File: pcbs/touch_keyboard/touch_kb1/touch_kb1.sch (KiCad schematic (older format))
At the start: 12 parts

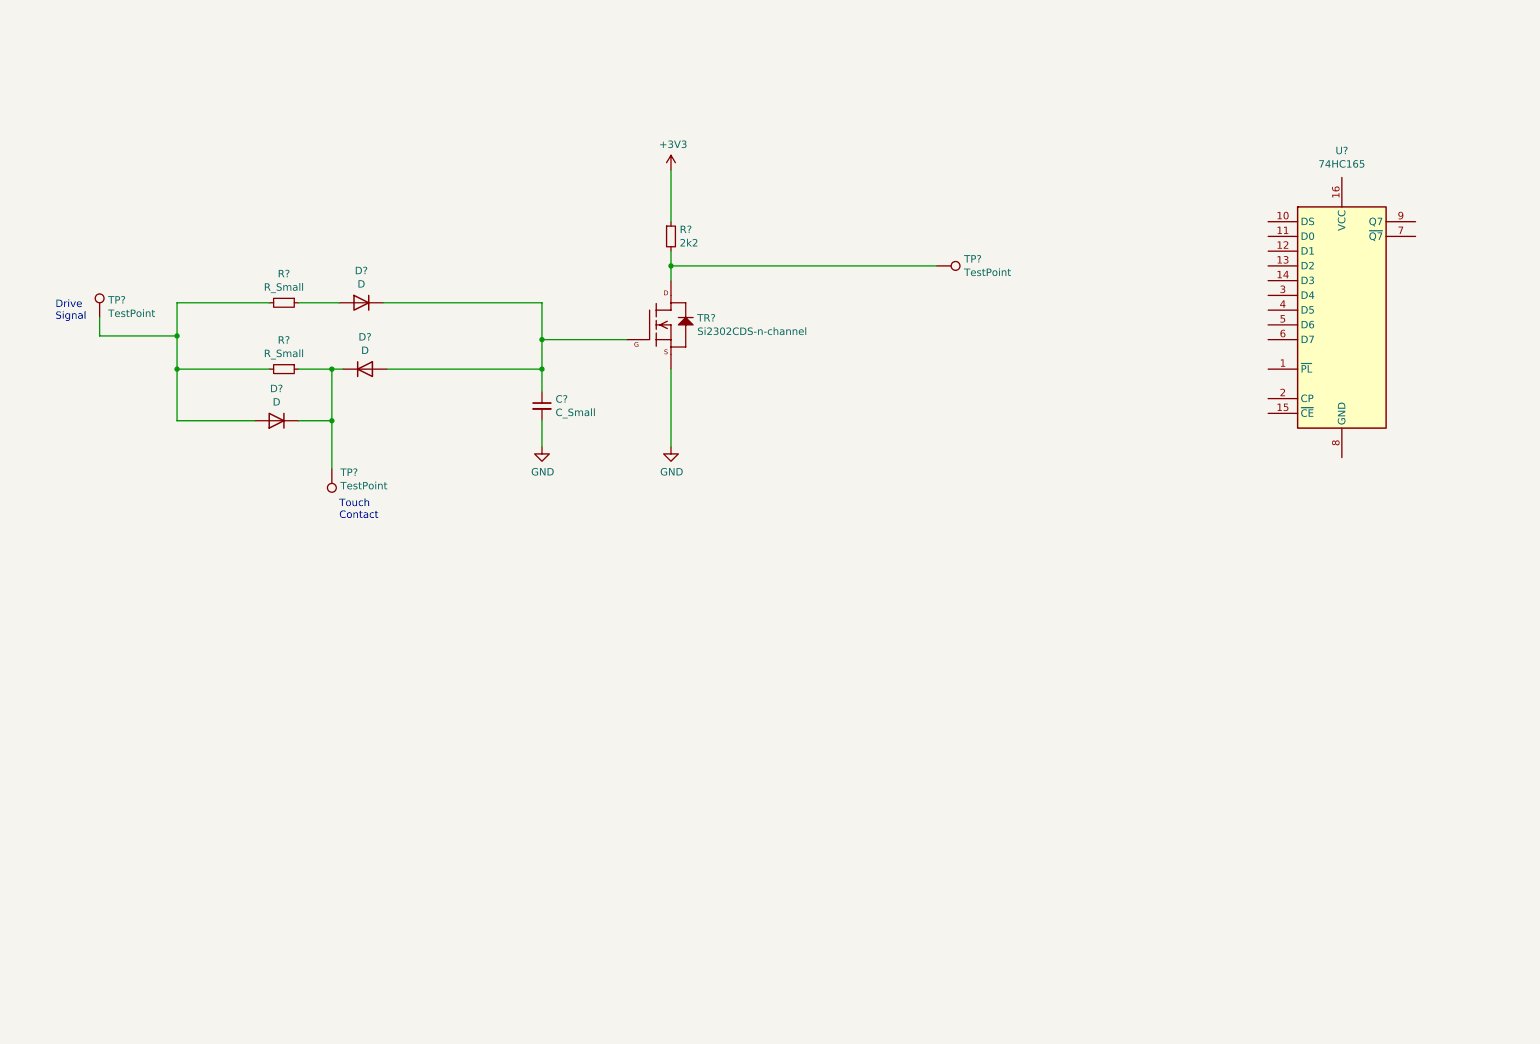
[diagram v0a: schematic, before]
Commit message: Updates
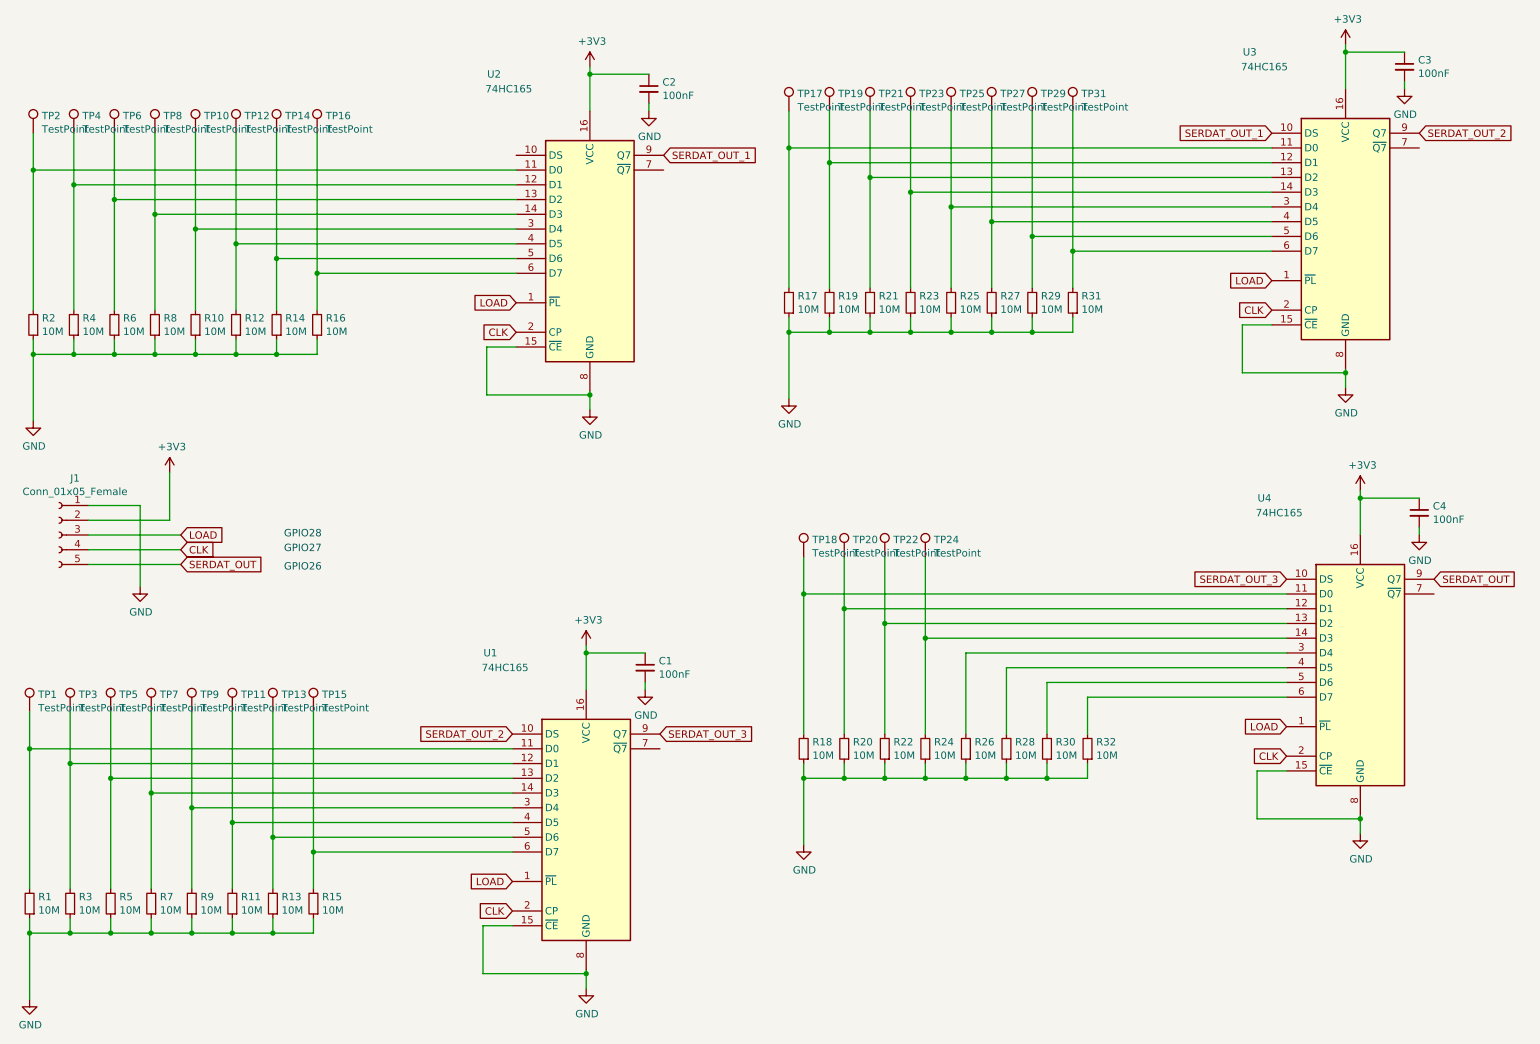
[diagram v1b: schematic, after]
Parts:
- removed C?: C_Small, symbol Device:C_Small
- removed D? (x3): D, symbol Device:D
- removed R? (x2): R_Small, symbol Device:R_Small
- removed TP? (x3): TestPoint, symbol Connector:TestPoint
- removed TR?: Si2302CDS-n-channel, Package_TO_SOT_SMD:SOT-23, symbol New_Library:Si2302CDS-n-channel
- added C1, C2, C3, C4: 100nF, Capacitor_SMD:C_0805_2012Metric_Pad1.18x1.45mm_HandSolder, symbol Device:C_Small
- added J1: Conn_01x05_Female, Connector_PinHeader_2.54mm:PinHeader_1x05_P2.54mm_Vertical_SMD_Pin1Left, symbol Connector:Conn_01x05_Female
- added R1, R10, R11, R12, R13, R14, R15, R16, R17, R18, R19, R2, R20, R21, R22, R23, R24, R25, R26, R27, R28, R29, R3, R30, R32, R4, R5, R6, R7, R8, R9: 10M, Resistor_SMD:R_0805_2012Metric_Pad1.20x1.40mm_HandSolder, symbol Device:R_Small
- added TP1, TP10, TP11, TP12, TP13, TP14, TP15, TP16, TP17, TP18, TP19, TP2, TP20, TP21, TP22, TP23, TP24, TP25, TP27, TP29, TP3, TP31, TP4, TP5, TP6, TP7, TP8, TP9: TestPoint, ajm_kicad:ESC_KB_Pad_half_size, symbol Connector:TestPoint
- added U1, U2, U4: 74HC165, Package_SO:SO-16_3.9x9.9mm_P1.27mm, symbol 74xx:74HC165
- R31: renamed from R?; value 2k2 -> 10M; footprint (none) -> Resistor_SMD:R_0805_2012Metric_Pad1.20x1.40mm_HandSolder
- U3: renamed from U?; footprint (none) -> Package_SO:SO-16_3.9x9.9mm_P1.27mm
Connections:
- net +3V3: now also U3.16 (VCC), C1.1, C2.1, C3.1, C4.1, J1.2 (Pin_2), U1.16 (VCC), U2.16 (VCC), U4.16 (VCC); no longer R31.1
- net GND: now also R31.1, U3.15 (~CE), U3.8 (GND), C1.2, C2.2, C3.2, C4.2, J1.1 (Pin_1), R1.1, R10.1, R11.1, R12.1, R13.1, R14.1, R15.1, R16.1, R17.1, R18.1, R19.1, R2.1, R20.1, R21.1, R22.1, R23.1, R24.1, R25.1, R26.1, R27.1, R28.1, R29.1, R3.1, R30.1, R32.1, R4.1, R5.1, R6.1, R7.1, R8.1, R9.1, U1.15 (~CE), U1.8 (GND), U2.15 (~CE), U2.8 (GND), U4.15 (~CE), U4.8 (GND)
- net at R31.2: now also U3.6 (D7), TP31.1
- net LOAD: now reaches U3.1 (~PL)
- net LOAD: now also J1.3 (Pin_3), U1.1 (~PL), U2.1 (~PL), U4.1 (~PL)
- net SERDAT_OUT_1: now reaches U3.10 (DS)
- net SERDAT_OUT_1: now also U2.9 (Q7)
- net at U3.11 (D0): now also R17.2, TP17.1
- net at U3.12 (D1): now also R19.2, TP19.1
- net at U3.13 (D2): now also R21.2, TP21.1
- net at U3.14 (D3): now also R23.2, TP23.1
- net CLK: now reaches U3.2 (CP)
- net CLK: now also J1.4 (Pin_4), U1.2 (CP), U2.2 (CP), U4.2 (CP)
- net at U3.3 (D4): now also R25.2, TP25.1
- net at U3.4 (D5): now also R27.2, TP27.1
- net at U3.5 (D6): now also R29.2, TP29.1
- net SERDAT_OUT_2: now reaches U3.9 (Q7)
- net SERDAT_OUT_2: now also U1.10 (DS)
- new net: R16.2, TP16.1, U2.6 (D7)
- new net: R2.2, TP2.1, U2.11 (D0)
- new net: R4.2, TP4.1, U2.12 (D1)
- new net: R6.2, TP6.1, U2.13 (D2)
- new net: R8.2, TP8.1, U2.14 (D3)
- new net: R10.2, TP10.1, U2.3 (D4)
- new net: R12.2, TP12.1, U2.4 (D5)
- new net: R14.2, TP14.1, U2.5 (D6)
- new net: R15.2, TP15.1, U1.6 (D7)
- new net: R1.2, TP1.1, U1.11 (D0)
- new net: R3.2, TP3.1, U1.12 (D1)
- new net: R5.2, TP5.1, U1.13 (D2)
- new net: R7.2, TP7.1, U1.14 (D3)
- new net: R9.2, TP9.1, U1.3 (D4)
- new net: R11.2, TP11.1, U1.4 (D5)
- new net: R13.2, TP13.1, U1.5 (D6)
- new net: R32.2, U4.6 (D7)
- new net: R18.2, TP18.1, U4.11 (D0)
- new net: R20.2, TP20.1, U4.12 (D1)
- new net: R22.2, TP22.1, U4.13 (D2)
- new net: R24.2, TP24.1, U4.14 (D3)
- new net: R26.2, U4.3 (D4)
- new net: R28.2, U4.4 (D5)
- new net: R30.2, U4.5 (D6)
- new net SERDAT_OUT: J1.5 (Pin_5), U4.9 (Q7)
- new net SERDAT_OUT_3: U1.9 (Q7), U4.10 (DS)
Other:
- note added: "GPIO26"
- note added: "GPIO27"
- note added: "GPIO28"
- note removed: "Drive\nSignal"
- note removed: "Touch\nContact"
- moved on the sheet: R31, U3
